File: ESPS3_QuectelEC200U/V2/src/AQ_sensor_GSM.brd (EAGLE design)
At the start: 110 x 64 mm, 100 parts, among them IC1 MIC29302WU, IC2 MCP73831/OT, J1 F-1X03-SIP-100-32, J3 PJ-002BH, Q1 MMBT2222, Q2 MMBT2222, Q3 MMBT2222, Q4 MMBT2222, Q5 MMBT2222, Q6 MMBT2222, Q7 MMBT2222, U1 LM7805S/NOPB, U3 TEXAS_INSTRUMENTS_LM1117IMP-3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, U5 TXS0108EPWR, X1 53048-08

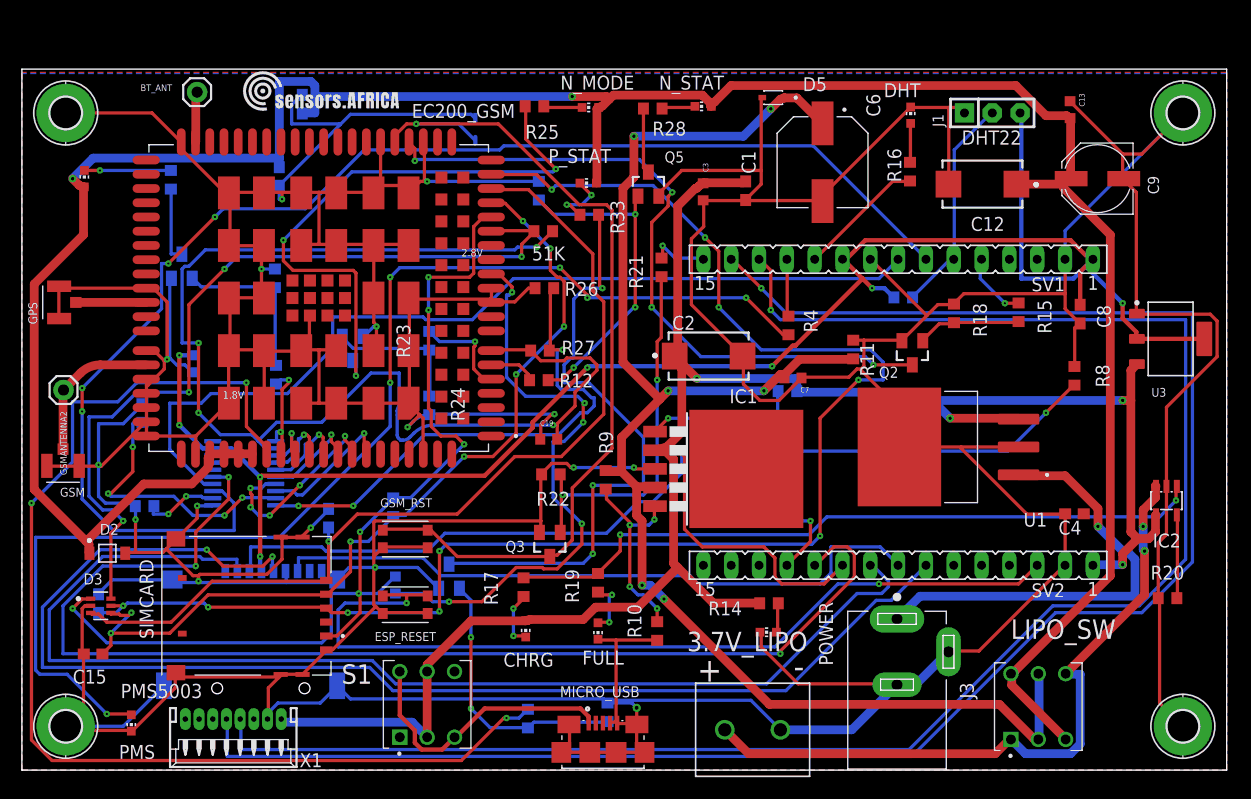
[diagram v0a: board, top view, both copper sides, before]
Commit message: V2 revised
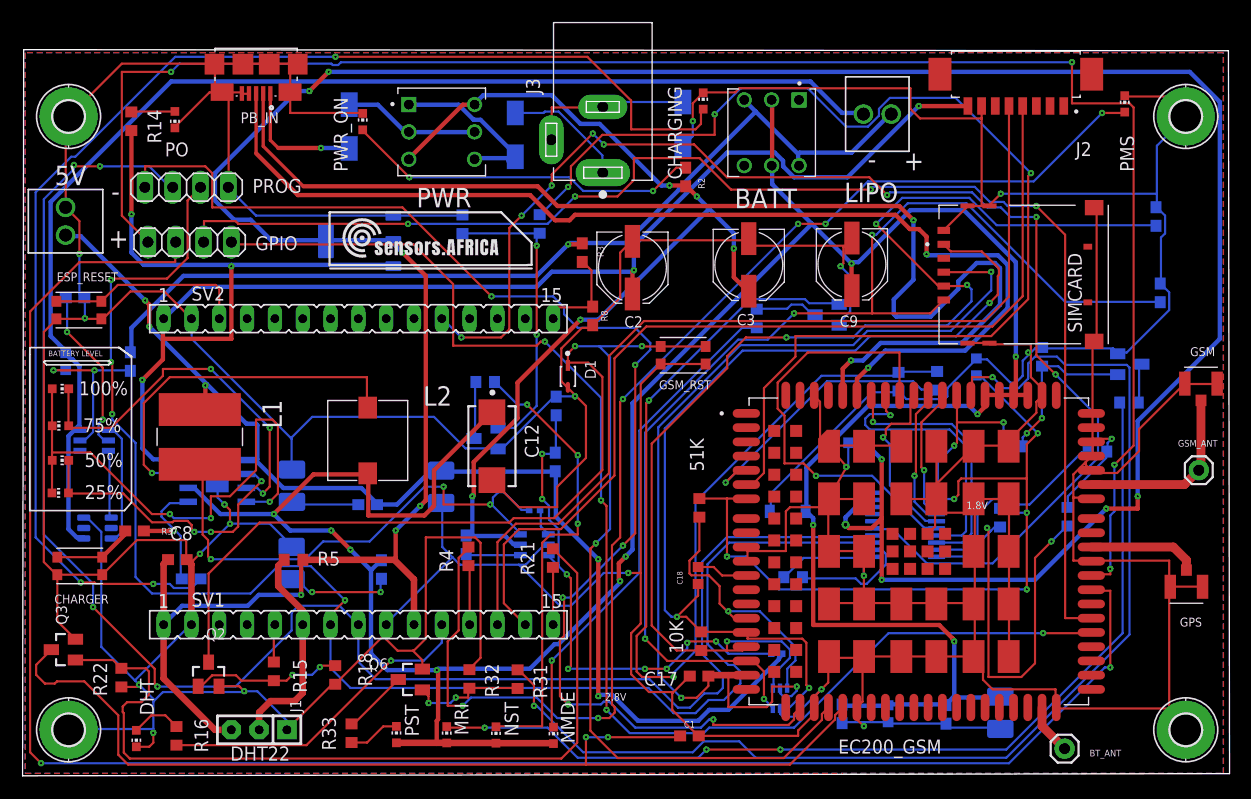
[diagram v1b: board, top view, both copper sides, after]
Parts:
- removed 3.7V_LIPO: 2828XX-2282837-2, Connector:TERMBLK_508-2N
- removed C6: EEEFN1C471P, EEEFN1C471P:CAP_EEEFN1C471P
- removed C7: 100nf, 06035C104K4T2A:CAPC1608X90N
- removed CHRG, POWER: RED, led:CHIP-LED0603
- removed D5: ESD56151W04, 4.7V TVS Diode:DIO_1N4148WS_RR
- removed FULL: YELLOW, led:CHIP-LED0603
- removed GSMANTENNA2: (no value), SparkFun-Connectors:1X01
- removed IC1: MIC29302WU, MIC29302WU:TO263-5
- removed IC2: MCP73831/OT, AQ_sensor_GSM:SOT23-5L
- removed LIPO_SW, S1: TL2285EE, TL2285EE:SW_TL2285EE
- removed MICRO_SD1: TF-01A, TF-01A:TF-01A
- removed MICRO_USB: 10118192-0001LF, AQ_sensor_GSM:AMPHENOL_10118192-0001LF
- removed M_RI, N_MODE, N_STAT, P_STAT: ORANGE, led:CHIP-LED0603
- removed Q1: MMBT2222, MMBT2222_:SOT23-BEC
- removed R11: 470R, rcl:R0603
- removed U1: LM7805S/NOPB, LM7805S_NOPB:TO254P1524X483-4N
- removed X1: 53048-08, AQ_sensor_GSM:53048-08
- added 100%, 25%, 50%, 75%, CHARGING, MRI, NMDE, NST, PST, PWR_ON: ORANGE, led:CHIP-LED0603
- added 5V, LIPO: 2828XX-2282834-2, Connector:TERMBLK_254-2N
- added BATT, PWR: TL2285EE, TL2285EE:SW_TL2285EE
- added C14: 22nF, SparkFun-Capacitors:0402-TIGHT
- added C21: 22pF, SparkFun-Capacitors:0402-TIGHT
- added C23, C24, C29, C30: TAJB106K016RNJ, Resistor_Capacitor:CAP_TANT_B
- added CHARGER: KMR621NGLFS, AQ_sensor_GSM:SW_KMR621NGLFS
- added D4, D6, D7: SS54-HF, SS54-HF schottkey Diode:DIOM5025X220N
- added DW01: DW01-P, DW01-P:SOT23-6L
- added GPIO, PROG: PINHD-1X4, Connector:1X04
- added GSM_ANT: (no value), SparkFun-Connectors:1X01
- added IP5306: IP5306, IP5306:SOIC127P600X165-9T209N
- added J2: 53261-0871, 53261-0871:MOLEX_53261-0871
- added L1: 784787047, Fixed Inductors:784787047
- added L2: 784778010, Fixed Inductors:784778010
- added MT2492: MT2492, MT2492:SOT95P280X145-6N
- added PB_IN: 10118192-0001LF, AQ_sensor_GSM:AMPHENOL_10118192-0001LF
- added PO: RED, led:CHIP-LED0603
- added Q8: FS8205, FS8205:SOT95P280X145-6N
- added R1: 110k, SparkFun-Resistors:0603
- added R37, R7: 10k, SparkFun-Resistors:0603
- added R6: 15k, SparkFun-Resistors:0603
- C1: value 10uF -> 10nF; device rcl:C0603 -> SparkFun-Capacitors:0603
- C2: value 470uf -> 100uF; device T495X477K010ATE100:CAPMP7343X430N -> rcl:PANASONIC_D
- C3: value 100nf -> 100uF; device 06035C104K4T2A:CAPC1608X90N -> rcl:PANASONIC_D
- C4: value 10uF -> 100nf; device rcl:C0603 -> 06035C104K4T2A:CAPC1608X90N
- R10: value 47K -> 100R; device rcl:R0603 -> SparkFun-Resistors:0603
- R16, R4: value 470 -> 470R
- R17, R19: value 470 -> 2R; device rcl:R0603 -> SparkFun-Resistors:0603
- R2: value 51K -> 1k; device rcl:R0603 -> SparkFun-Resistors:0603
- R20: value 2K -> 220R; device rcl:R0603 -> SparkFun-Resistors:0603
- R3: value 4.7K -> 47k; device rcl:R0603 -> SparkFun-Resistors:0603
- R8: value 47K -> 10k; device rcl:R0603 -> SparkFun-Resistors:0603
- R9: value 100k -> 1k; device rcl:R0603 -> SparkFun-Resistors:0603
- moved H3 116.7 mm to (106.3, 3.68), turned to 180 degrees
- moved H4 116.4 mm to (106.3, 59.7), turned to 180 degrees
- moved H2 116.3 mm to (4.26, 3.68), turned to 180 degrees
- moved H1 116.0 mm to (4.26, 59.7), turned to 180 degrees
- moved PMS 106.9 mm to (100.7, 60.8), turned to 0 degrees
- moved GPS 106.1 mm to (106.3, 16.7), turned to 180 degrees
- moved C15 104.9 mm to (103.5, 50.5), flipped to the bottom, turned to 90 degrees
- moved GSM 104.2 mm to (107.7, 35.3), turned to 0 degrees
- moved BT_ANT 99.3 mm to (95.2, 1.96), turned to 180 degrees
- moved C4 93.1 mm to (4.00, 37.3), flipped to the bottom, turned to 90 degrees
- moved DHT 90.8 mm to (10.4, 2.88), turned to 180 degrees
- moved R36 89.8 mm to (101.1, 33.6), turned to 0 degrees
- moved R20 89.2 mm to (15.5, 17.5), flipped to the bottom, turned to 0 degrees
- moved J1 87.5 mm to (21.7, 3.68), turned to 180 degrees
- moved R30 87.3 mm to (98.2, 29.1), turned to 180 degrees
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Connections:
- net USB_VBUS renamed G_USB_VBUS
- removed net +5V: C1.1, C2.1, C3.2, CHRG.A, IC1.2, IC2.4, R14.2, R2.2, S1.2, S1.5, SV2.1, U1.3, U3.3, X1.8
- removed net BP: 3.7V_LIPO.2, IC2.3, LIPO_SW.1, LIPO_SW.6
- removed net CP: C6.1, C7.2, D5.C, IC1.4, LIPO_SW.2, LIPO_SW.5, R11.2, R9.2
- removed net D+: MICRO_USB.3
- removed net D-: MICRO_USB.2
- removed net JACKP: J3.1, U1.1
- removed net N$12: FULL.A, R19.1
- removed net N$36: Q1.B, R3.2
- removed net N$38: IC1.5, R10.2, R9.1
- removed net TF-CLK: MICRO_SD1.5, SV2.7
- removed net TF-CS: MICRO_SD1.2, SV2.9
- removed net TF-MISO: MICRO_SD1.7, SV2.8
- removed net TF-MOSI: MICRO_SD1.3, SV2.10
- removed net USBP: MICRO_USB.1, S1.3, S1.4
- removed net VRTC: C4.1
- new net 4.5-16V: C3.+, MT2492.5, PWR.3, PWR.4, R2.1, R7.2
- new net 5VT: D4.1, PWR.2, PWR.5
- new net 5V_IN: 5V.1, C21.1, C30.1, IP5306.1, L1.2, R1.2, R17.2
- new net 5V_OUT: C2.+, IP5306.8, J2.8, R14.2, SV2.1, U3.3
- new net BATT-: C4.2, DW01.6, LIPO.2, Q8.1
- new net BMSV: R3.2, R8.1, SV2.15
- new net G_ADC0: EC200_GSM.45, GPIO.1
- new net G_ADC1: EC200_GSM.44, GPIO.2
- new net G_ADC2: EC200_GSM.43
- new net G_GPIO1: EC200_GSM.126
- new net G_I2C_SCL: EC200_GSM.41, GPIO.4
- new net G_I2C_SDA: EC200_GSM.42, GPIO.3
- new net G_SPI_CLK: EC200_GSM.40
- new net G_SPI_CS: EC200_GSM.37
- new net G_SPI_MISO: EC200_GSM.39
- new net G_SPI_MOSI: EC200_GSM.38
- new net G_USB_BOOT: EC200_GSM.115, PROG.1
- new net G_USB_D+: EC200_GSM.69, PB_IN.3
- new net G_USB_D-: EC200_GSM.70, PB_IN.2
- new net LBV: BATT.3, BATT.4, LIPO.1, R10.2, R3.1
- new net N$10: C21.2, MT2492.3, R1.1, R6.2
- new net N$11: MT2492.4, R7.1
- new net N$14: 100%.A, 25%.C, 50%.A, 75%.C, IP5306.4
- new net N$17: 25%.A, 50%.C, IP5306.2
- new net N$18: 100%.C, 75%.A, IP5306.3
- new net N$19: DW01.3, Q8.4
- new net N$20: CHARGER.1_1, CHARGER.1_2, R37.1
- new net N$21: IP5306.7, L2.1
- new net N$24: C24.1, R19.1
- new net N$3: C14.1, MT2492.1
- new net N$45: IP5306.5, R20.2, R37.2
- new net N$46: CHARGING.A, R20.1
- new net N$47: DW01.2, R9.1
- new net N$59: D4.2, PB_IN.1
- new net N$60: D7.1, J3.2, J3.3
- new net N$61: D6.2, J3.1
- new net VUSB: D6.1, PWR.1, PWR.6
- net +3V3: no longer MICRO_SD1.4
- net GND: now also 5V.2, C2.-, C23.2, C24.2, C29.2, C3.-, C30.2, CHARGER.2_1, CHARGER.2_2, CHARGING.C, D1.2, D7.2, IP5306.9, J2.7, MT2492.2, PB_IN.4, PB_IN.5, PB_IN.SH1, PB_IN.SH2, PB_IN.SH3, PB_IN.SH4, PB_IN.SH5, PB_IN.SH6, PO.C, PROG.4, PWR_ON.C, Q8.3, R6.1, R8.2, R9.2; no longer 3.7V_LIPO.1, C2.2, C3.1, C4.2, C6.2, C7.1, D1.1, D5.A, FULL.C, IC1.3, IC2.2, J3.2, J3.3, MICRO_SD1.6, MICRO_SD1.MP1, MICRO_SD1.MP2, MICRO_SD1.MP3, MICRO_SD1.MP4, MICRO_USB.4, MICRO_USB.5, MICRO_USB.SH1, MICRO_USB.SH2, MICRO_USB.SH3, MICRO_USB.SH4, MICRO_USB.SH5, MICRO_USB.SH6, POWER.C, R10.1, R11.1, R20.2, R8.1, U1.2, U1.4, X1.7
- net GSM_ANT: now also GSM_ANT.1; no longer GSMANTENNA2.1
- net GSM_RST: now also D1.1, GSM_RST.2_1, GSM_RST.2_2
- net MCU_RXD: now also PROG.2
- net MCU_TXD: now also PROG.3
- net N$13: now also C23.1, R17.1; no longer IC2.5, R20.1
- net N$25: now also PO.A; no longer POWER.A
- net N$30: now also NMDE.C; no longer N_MODE.C
- net N$34: now also NST.C; no longer N_STAT.C
- net N$35: now also PWR_ON.A, R2.2; no longer IC1.1, Q1.C, R2.1
- net N$37: now also C4.1, DW01.5, R10.1; no longer Q1.E, R8.2
- net N$39: now also PST.C; no longer P_STAT.C
- net N$44: now also MRI.C; no longer M_RI.C
- net N$6: now also C14.2, L1.1, MT2492.6; no longer CHRG.C, R17.1
- net N$9: now also DW01.1, Q8.6; no longer IC2.1, R17.2, R19.2
- net PMS_RX: now also J2.5; no longer X1.5
- net PMS_TX: now also J2.4; no longer X1.4
- net PWRKEY: now also C1.1; no longer D1.2, GSM_RST.2_1, GSM_RST.2_2
- net VBAT_EN: no longer R3.1
- net V_LIPO: now also BATT.2, BATT.5, C29.1, IP5306.6, L2.2, MRI.A, NMDE.A, NST.A, PST.A, R19.2; no longer LIPO_SW.3, LIPO_SW.4, M_RI.A, N_MODE.A, N_STAT.A, P_STAT.A
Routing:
- net +5V: track 177.2 -> 0.00 mm, vias 4 -> 0
- net G_ADC1: track 0.00 -> 168.6 mm, vias 0 -> 2
- net G_ADC0: track 0.00 -> 158.6 mm, vias 0 -> 4
- net 5V_OUT: track 0.00 -> 153.0 mm, vias 0 -> 5
- net CP: track 135.6 -> 0.00 mm, vias 6 -> 0
- net +3V3: track 161.4 -> 286.9 mm, vias 8 -> 11
- net G_I2C_SDA: track 0.00 -> 124.8 mm, vias 0 -> 4
- net G_I2C_SCL: track 0.00 -> 121.0 mm, vias 0 -> 4
- net N$46: track 0.00 -> 120.6 mm, vias 0 -> 3
- net G_USB_BOOT: track 0.00 -> 118.2 mm, vias 0 -> 6
- net TF-CLK: track 117.3 -> 0.00 mm, vias 2 -> 0
- net BATT-: track 0.00 -> 113.7 mm
- net G_USB_D-: track 0.00 -> 111.3 mm, vias 0 -> 2
- net TF-CS: track 109.0 -> 0.00 mm
- net 5V_IN: track 0.00 -> 105.8 mm, vias 0 -> 5
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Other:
- board size 110 x 64 mm -> 110.2 x 66.3 mm
- board text added: "BATTERY LEVEL"
- board text removed: "/Users/augustinemwendwa/Downloads/Logo-Files-01 (2) (1) (1).bmp"
- board text removed: "/Users/augustinemwendwa/Downloads/Logo-Files-01 (2) (1).bmp"
- board text removed: "PMS5003"
